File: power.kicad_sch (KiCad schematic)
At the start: 22 parts, among them J1 Conn_01x06_Pin, U13 LP5907MFX-3.0, U14 LP5907MFX-4.5, U3 LM66100DCK, U4 LP5907MFX-3.0, U5 TPS22918TDBVRQ1, U6 LP5907MFX-3.0

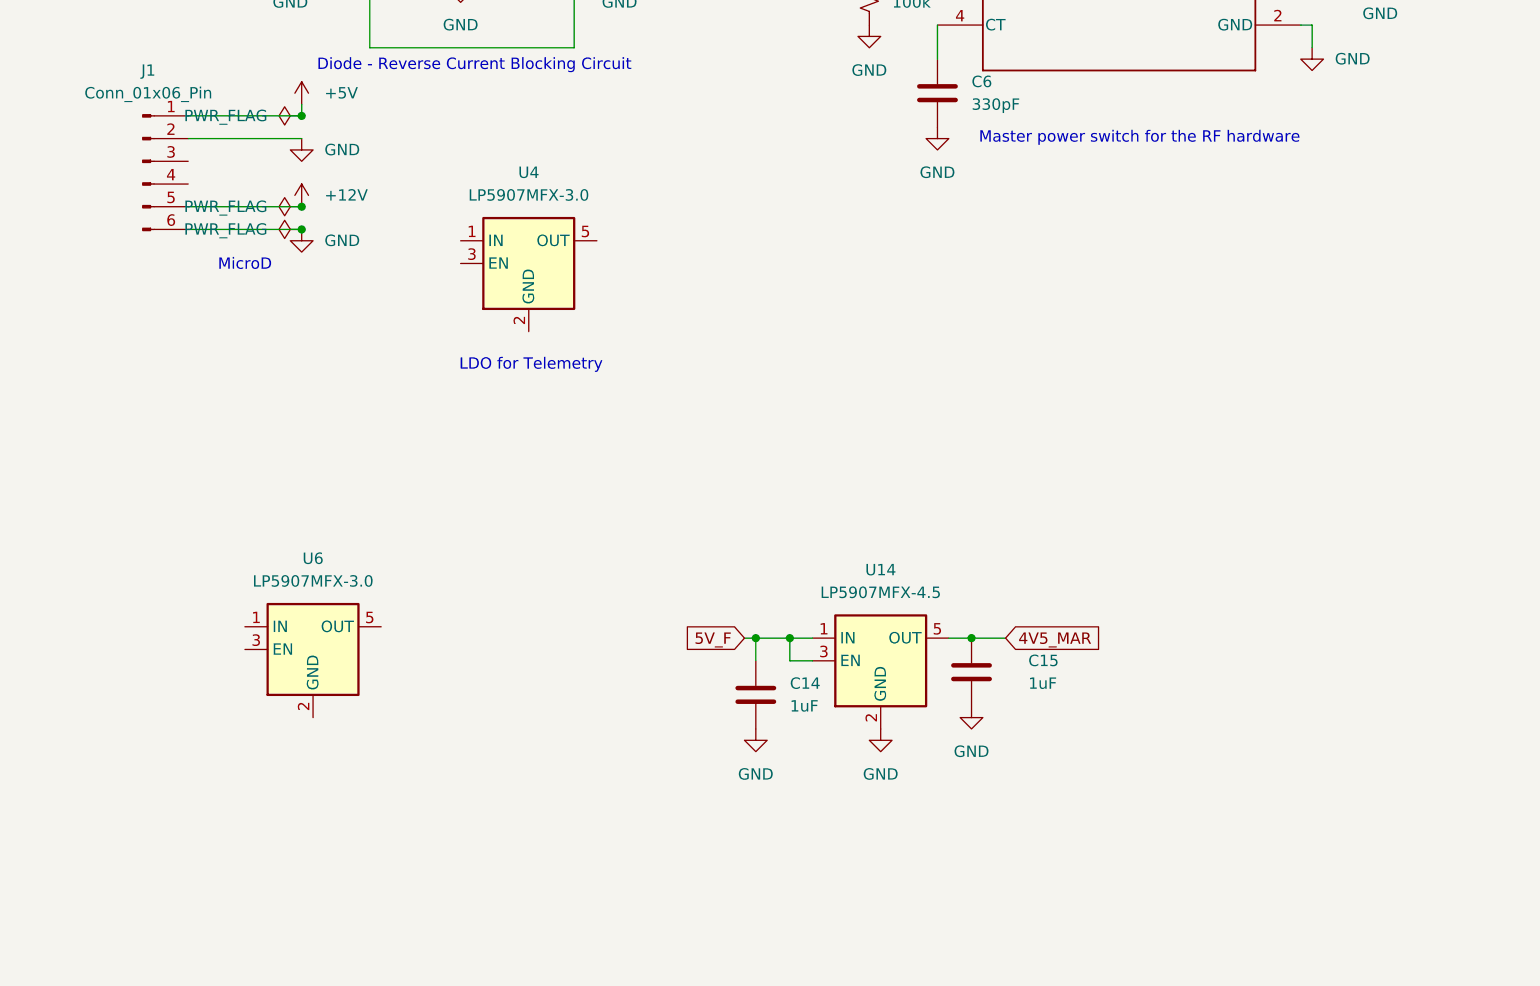
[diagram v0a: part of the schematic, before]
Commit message: LDO wiring
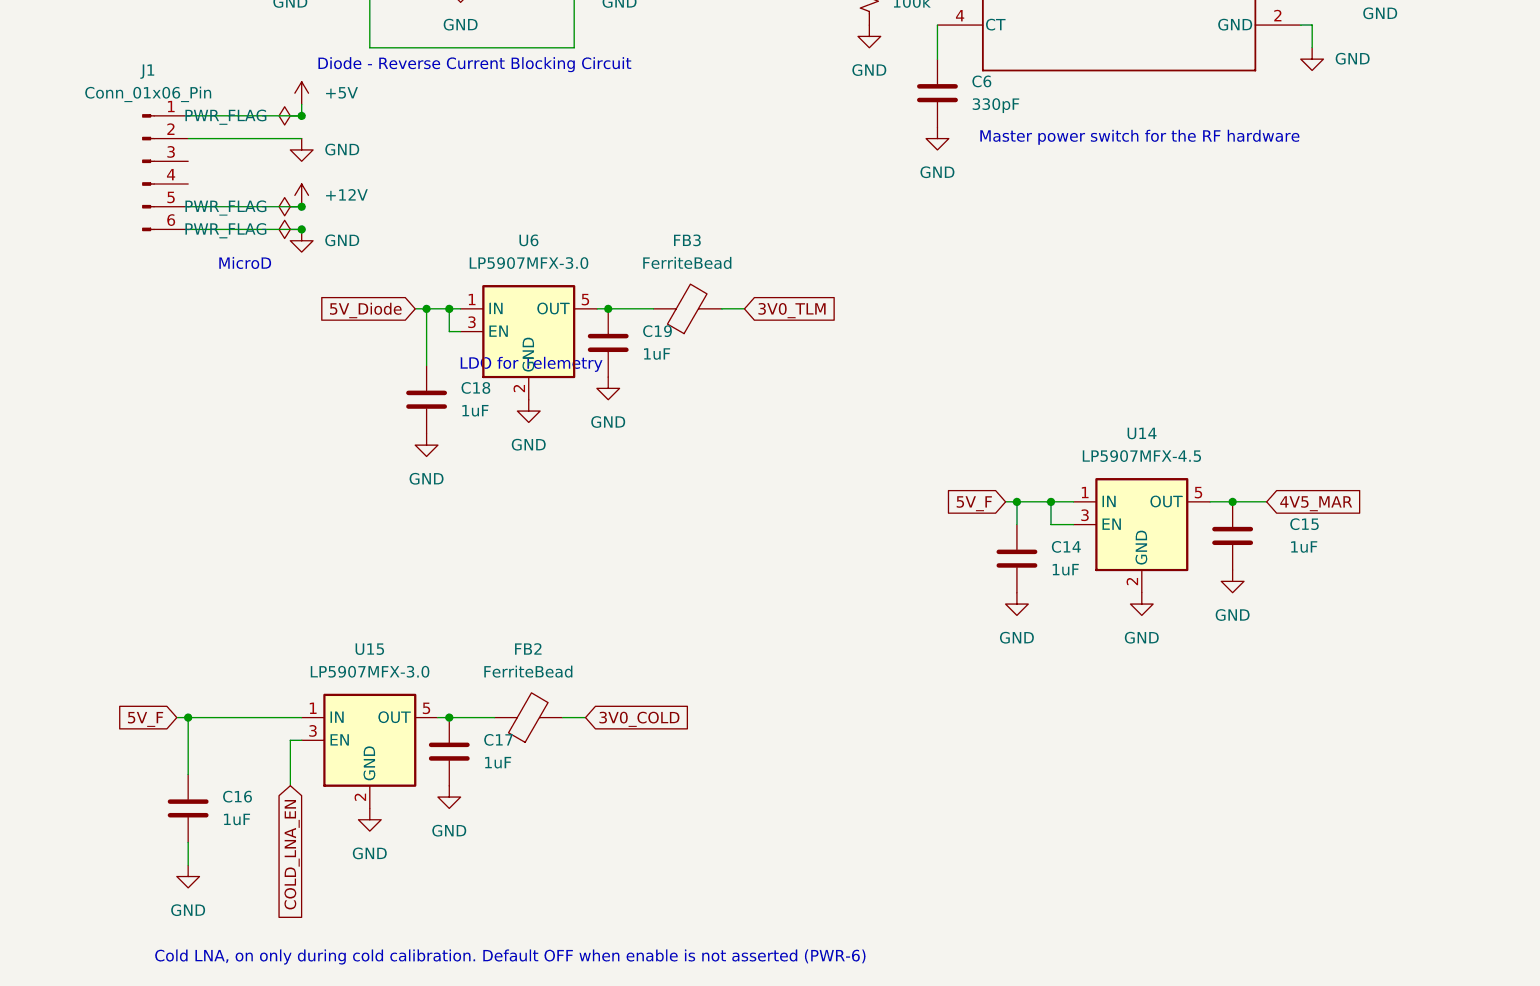
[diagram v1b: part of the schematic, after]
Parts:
- removed U4: LP5907MFX-3.0, Package_TO_SOT_SMD:SOT-23-5, symbol Regulator_Linear:LP5907MFX-3.0
- added C16, C17, C18, C19: 1uF, symbol Device:C
- added FB2, FB3: FerriteBead, symbol Device:FerriteBead
- added U15: LP5907MFX-3.0, Package_TO_SOT_SMD:SOT-23-5, symbol Regulator_Linear:LP5907MFX-3.0
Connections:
- net 5V_Diode: now also U6.1 (IN), U6.3 (EN), C18.1
- net 5V_F: now also C16.1, U15.1 (IN)
- net GND: now also U6.2 (GND), C16.2, C17.2, C18.2, C19.2, U15.2 (GND)
- net at U6.5 (OUT): now also C19.1, FB3.1
- new net: C17.1, FB2.1, U15.5 (OUT)
- new net 3V0_COLD: FB2.2
- new net 3V0_TLM: FB3.2
- new net COLD_LNA_EN: U15.3 (EN)
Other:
- note added: "Cold LNA, on only during cold calibration. Default OFF when enable is not asserted (PWR-6)"
- moved on the sheet: C14, C15, U14
